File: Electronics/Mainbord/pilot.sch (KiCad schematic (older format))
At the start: 26 parts, among them J10 Screw_Terminal_01x10, J11 Screw_Terminal_01x10, J12 Screw_Terminal_01x10, J13 Screw_Terminal_01x10, J14 Screw_Terminal_01x10, J15 Screw_Terminal_01x02, U10 74HC165, U11 74HC165, U12 74HC165, U13 74HC165, U14 74HC595, U15 74HC4051, U9 74HC165

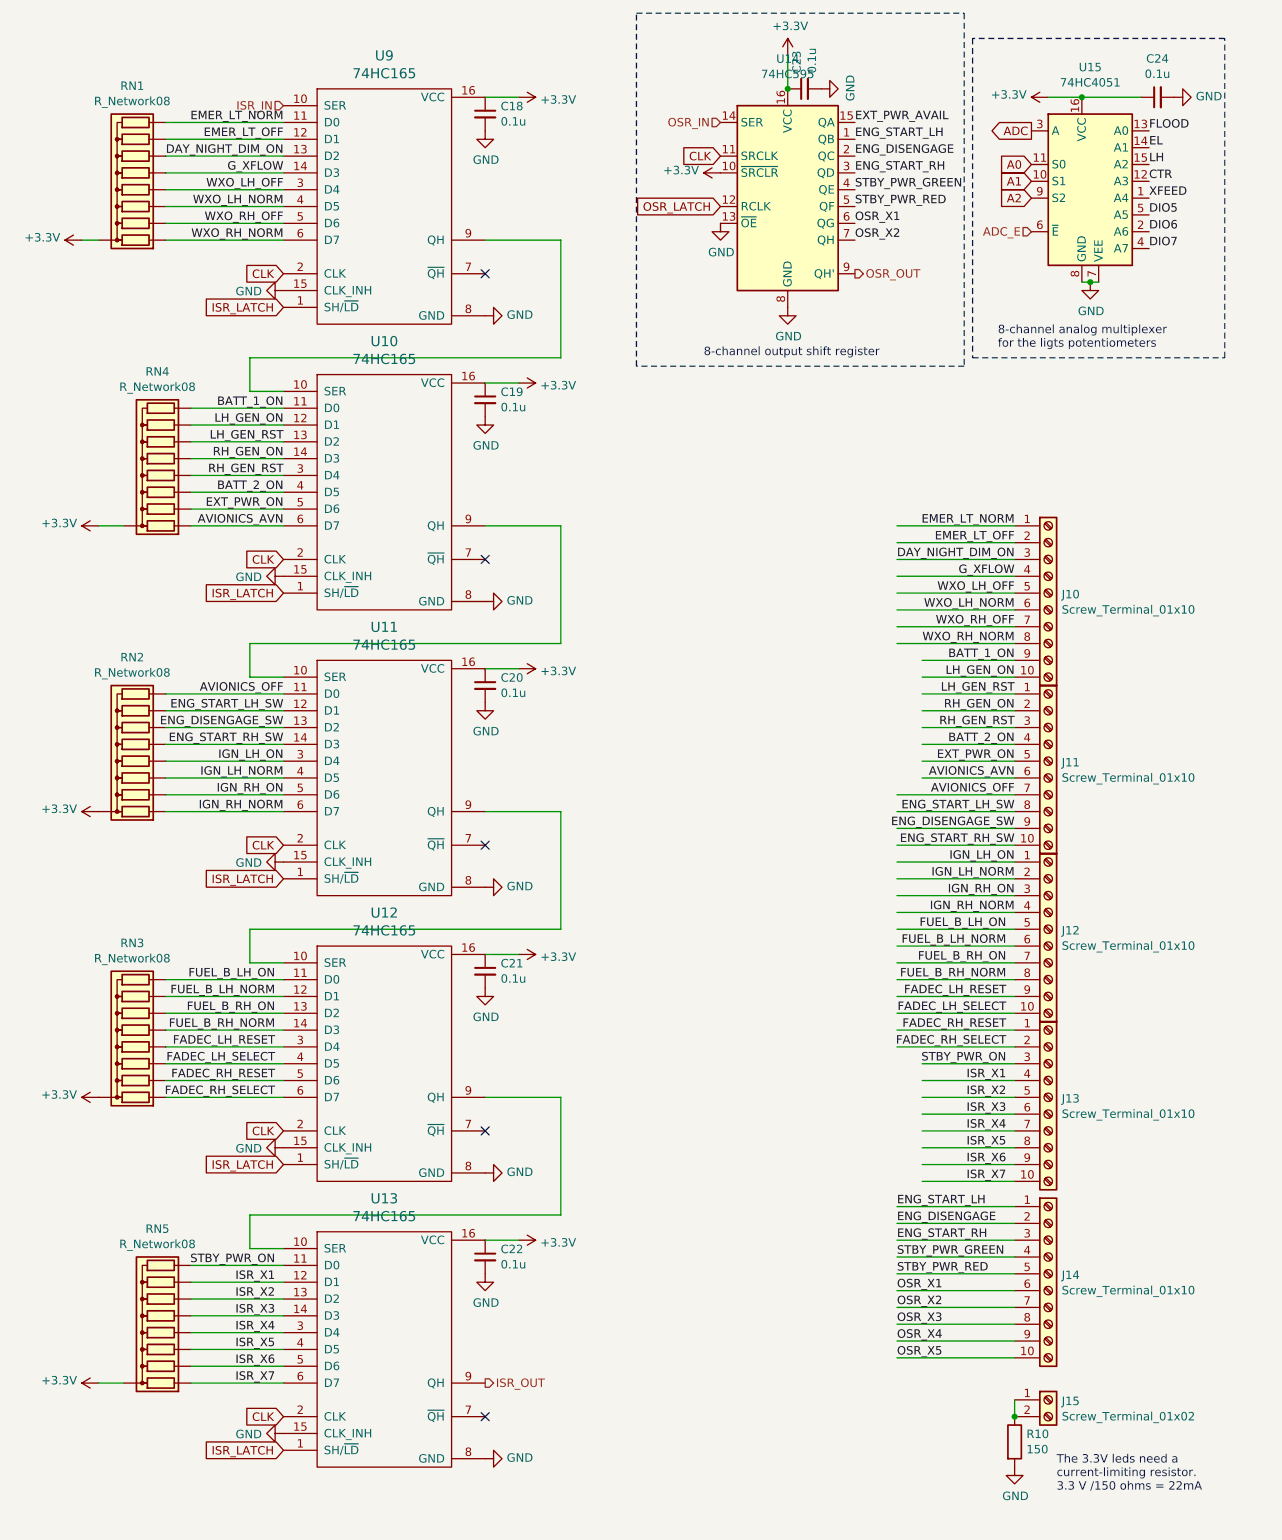
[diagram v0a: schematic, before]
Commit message: Electronics - Misc works
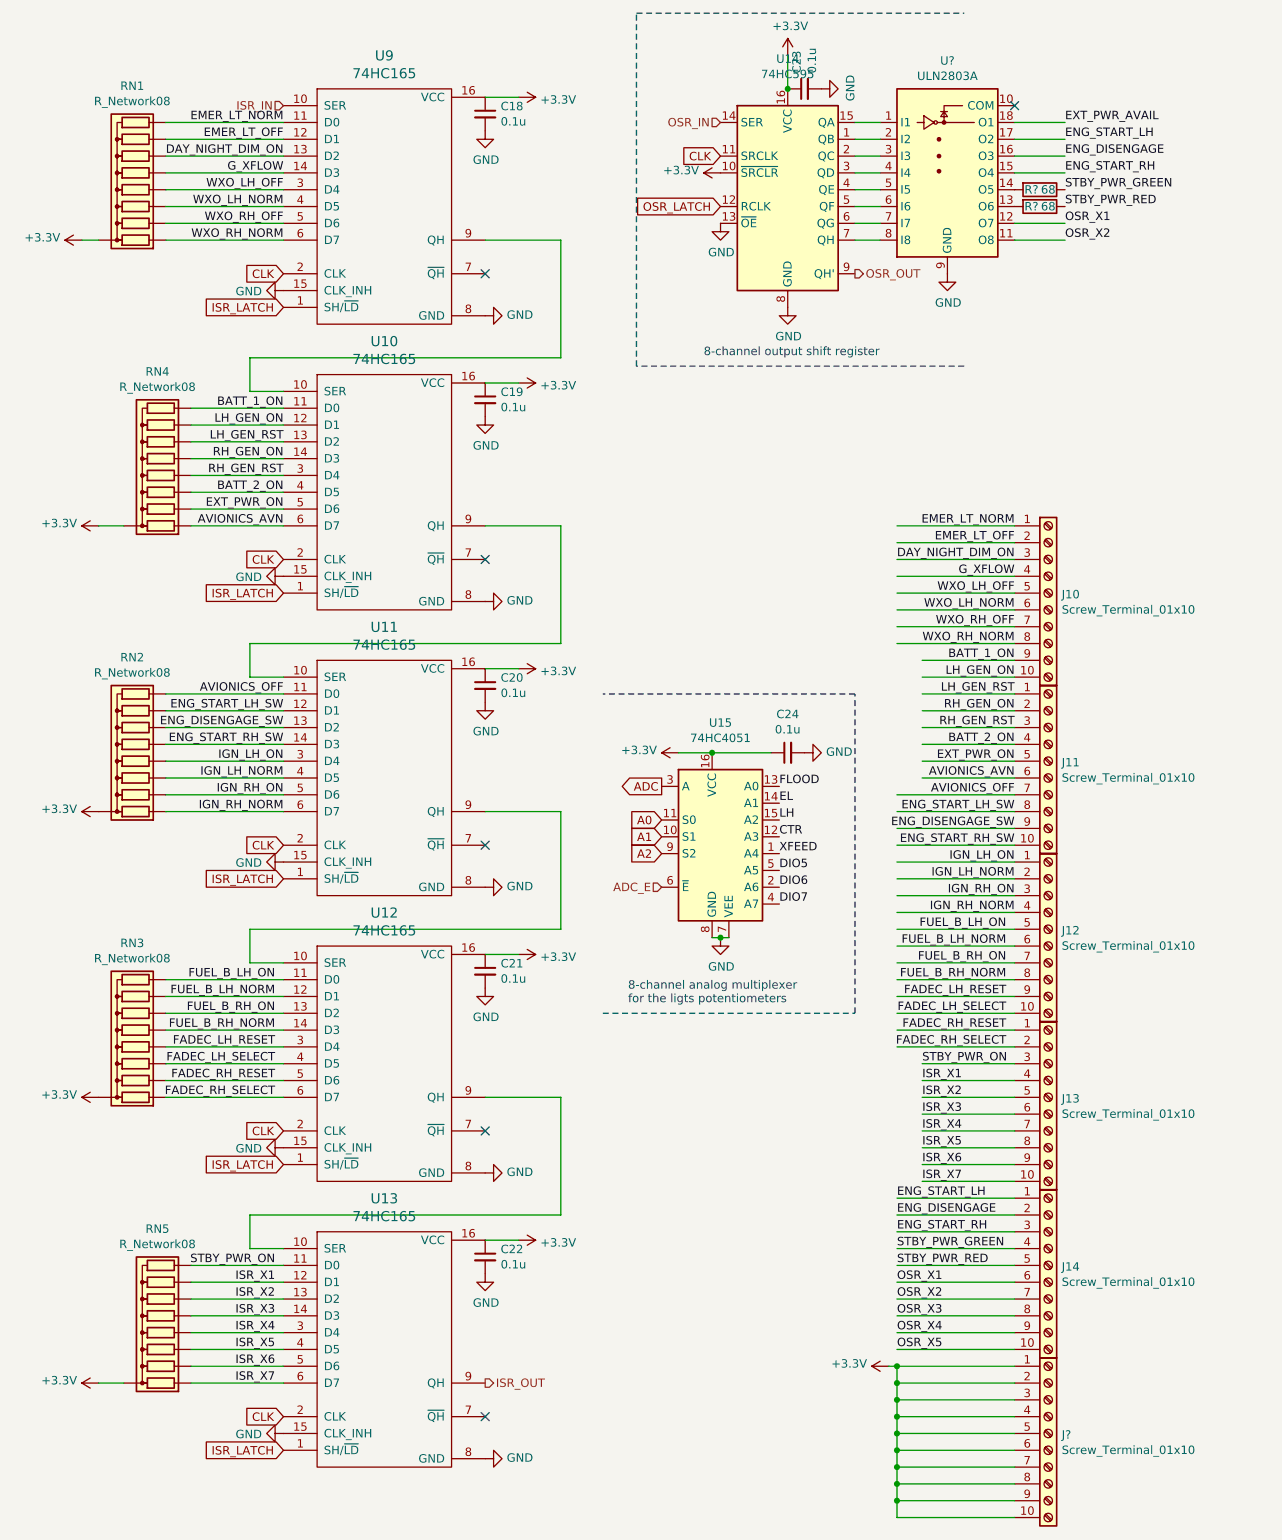
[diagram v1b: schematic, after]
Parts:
- removed J15: Screw_Terminal_01x02, symbol Connector:Screw_Terminal_01x02
- removed R10: 150, symbol Device:R
- added J?: Screw_Terminal_01x10, symbol Connector:Screw_Terminal_01x10
- added R? (x2): 68, symbol Device:R
- added U?: ULN2803A, symbol Transistor_Array:ULN2803A
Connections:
- wire segments 124 -> 157
- no-connect marks 5 -> 6
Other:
- note removed: "The 3.3V leds need a \ncurrent-limiting resistor.\n3.3 V /150 ohms = 22mA\n"
- moved on the sheet: C24, J14, U15
